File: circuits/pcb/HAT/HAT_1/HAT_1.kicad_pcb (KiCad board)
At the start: 2 copper layers, 75.4 x 55.9 mm, 11 parts, among them J1 Raspberry pi 5 GPIOs, J12 power input, J2 motor1, J3 motor1, J4 Conn_01x16_Pin, J5 motor2, J7 motor2, U1 ESP32-DEVKITC-32D, U2 L293D, U3 L293D

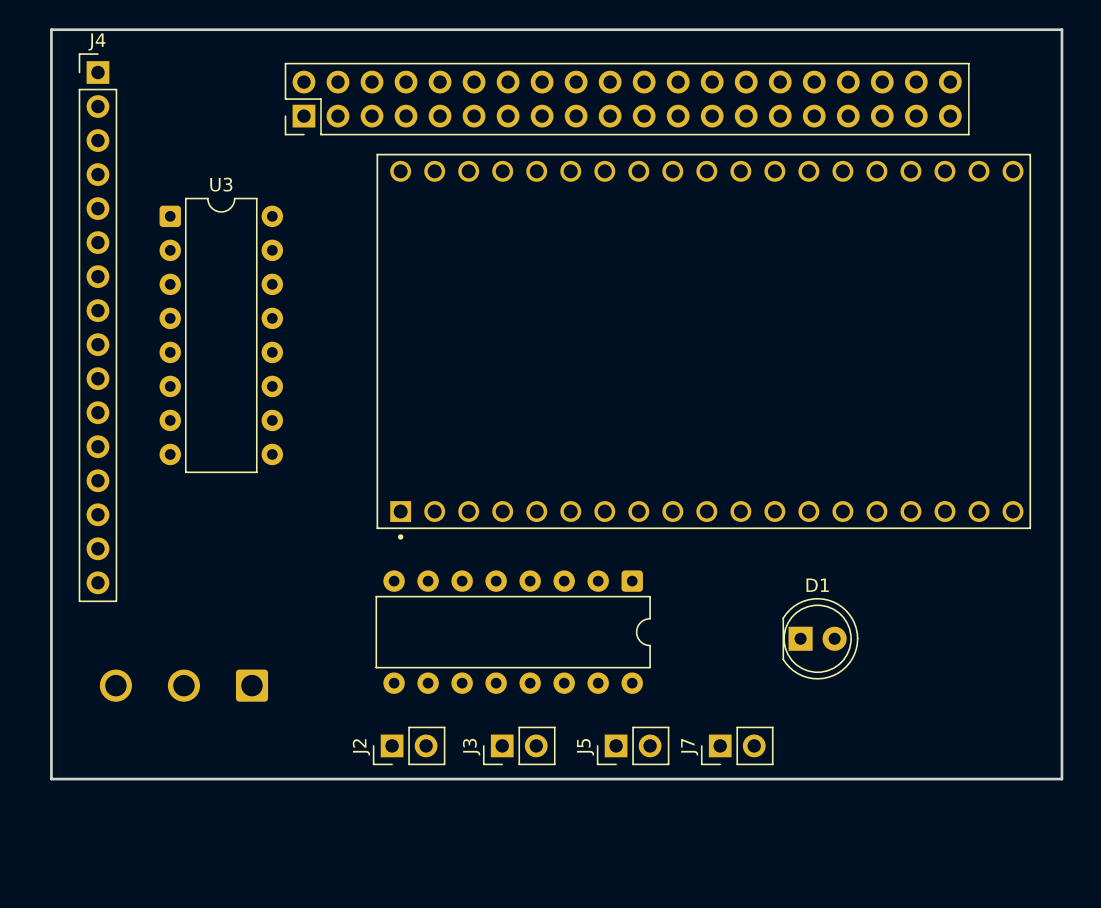
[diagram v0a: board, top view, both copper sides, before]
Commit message: ..
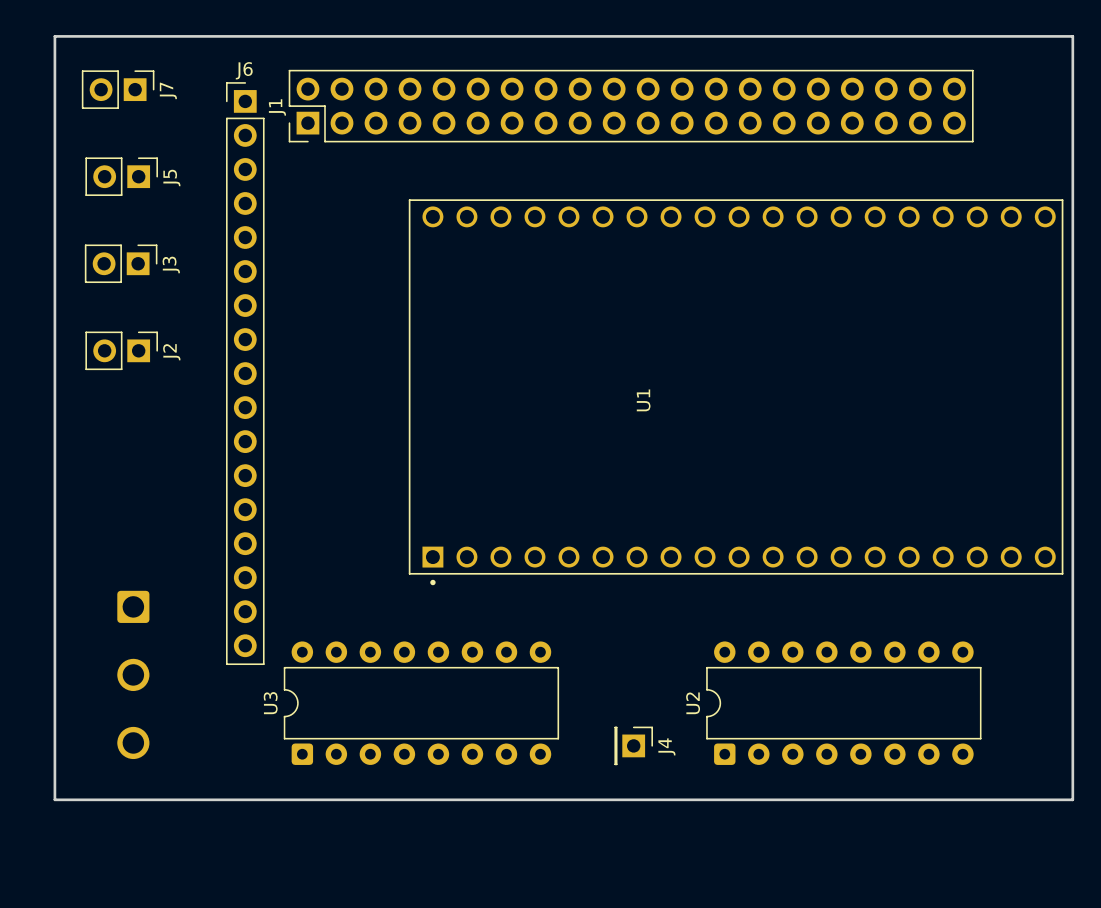
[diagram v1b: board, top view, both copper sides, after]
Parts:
- removed D1: LED, LED_THT:LED_D5.0mm
- added J6: Conn_01x17_Pin, Connector_PinHeader_2.54mm:PinHeader_1x17_P2.54mm_Vertical, F.Cu at (121.0, 79.9)
- J4: value Conn_01x16_Pin -> Conn_01x01_Pin; footprint Connector_PinHeader_2.54mm:PinHeader_1x16_P2.54mm_Vertical -> Connector_PinHeader_2.54mm:PinHeader_1x01_P2.54mm_Vertical
- moved J7 65.6 mm to (112.8, 79.0), turned to -90 degrees
- moved J4 64.2 mm to (150.0, 128.0), turned to -90 degrees
- moved J5 55.5 mm to (113.0, 85.5), turned to -90 degrees
- moved J3 45.1 mm to (113.0, 92.0), turned to -90 degrees
- moved U3 41.4 mm to (125.3, 128.6), turned to 90 degrees
- moved J2 35.0 mm to (113.0, 98.5), turned to -90 degrees
- moved U2 14.7 mm to (156.8, 128.6), turned to 90 degrees
- moved J12 10.6 mm to (112.6, 117.6), turned to -90 degrees
- moved U1 4.17 mm to (154.8, 101.2)
- moved J1 0.60 mm to (125.7, 81.5)
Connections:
- J4 pad 1: +5V -> Net-(J4-Pin_1)
- U1 pad J2-1: unconnected-(U1-3V3-PadJ2-1) -> Net-(J4-Pin_1)
- U1 pad J3-11: GPS RX -> TH_CAM SDA
- U1 pad J3-16: Net-(D1-A) -> TH_CAM SCL
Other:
- board size 75.4 x 55.9 mm -> 76 x 57 mm

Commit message: ...
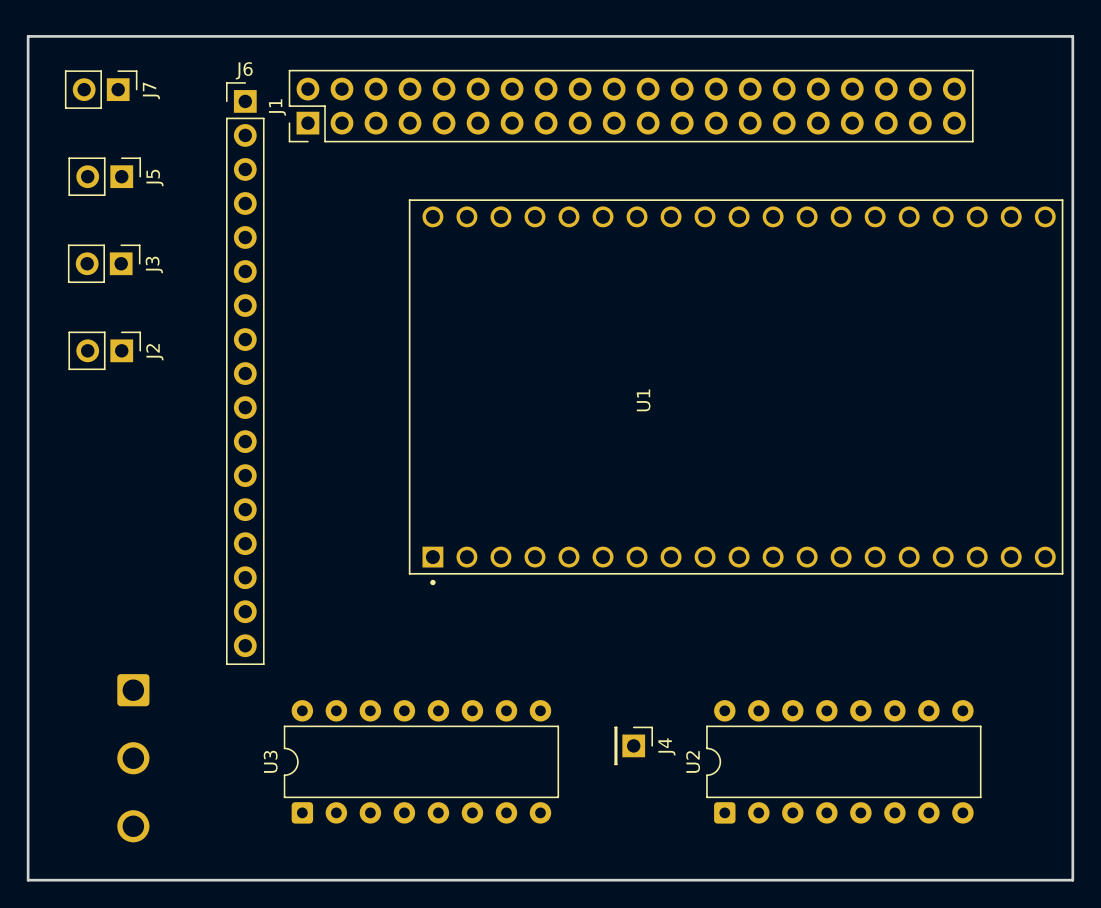
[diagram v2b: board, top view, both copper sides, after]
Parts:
- moved J12 6.22 mm to (112.6, 123.8)
- moved U2 4.38 mm to (156.8, 133.0)
- moved U3 4.38 mm to (125.3, 133.0)
- moved J2 1.27 mm to (111.8, 98.5)
- moved J3 1.27 mm to (111.7, 92.0)
- moved J5 1.27 mm to (111.8, 85.5)
- moved J7 1.27 mm to (111.5, 79.0)
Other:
- board size 76 x 57 mm -> 78 x 63 mm
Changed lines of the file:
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@@
 	(footprint "Package_DIP:DIP-16_W7.62mm"
 		(layer "F.Cu")
-		(at 156.8 128.62 90)
+		(at 156.8 133 90)
 		(descr "16-lead though-hole mounted DIP package, row spacing 7.62mm (300 mils)")
 		(tags "THT DIP DIL PDIP 2.54mm 7.62mm 300mil")
@@
 	(footprint "Connector_PinHeader_2.54mm:PinHeader_1x02_P2.54mm_Vertical"
 		(layer "F.Cu")
-		(at 113.04 85.5 -90)
+		(at 111.775 85.5 -90)
 		(descr "Through hole straight pin header, 1x02, 2.54mm pitch, single row")
 		(tags "Through hole pin header THT 1x02 2.54mm single row")
@@
 	(footprint "Connector_PinHeader_2.54mm:PinHeader_1x02_P2.54mm_Vertical"
 		(layer "F.Cu")
-		(at 113.04 98.5 -90)
+		(at 111.775 98.5 -90)
 		(descr "Through hole straight pin header, 1x02, 2.54mm pitch, single row")
 		(tags "Through hole pin header THT 1x02 2.54mm single row")
@@
 	(footprint "Package_DIP:DIP-16_W7.62mm"
 		(layer "F.Cu")
-		(at 125.26 128.62 90)
+		(at 125.26 133 90)
 		(descr "16-lead though-hole mounted DIP package, row spacing 7.62mm (300 mils)")
 		(tags "THT DIP DIL PDIP 2.54mm 7.62mm 300mil")
@@
 	(footprint "Connector_PinHeader_2.54mm:PinHeader_1x02_P2.54mm_Vertical"
 		(layer "F.Cu")
-		(at 112.775 79 -90)
+		(at 111.51 79 -90)
 		(descr "Through hole straight pin header, 1x02, 2.54mm pitch, single row")
 		(tags "Through hole pin header THT 1x02 2.54mm single row")
@@
 	(footprint "Connector_PinHeader_2.54mm:PinHeader_1x02_P2.54mm_Vertical"
 		(layer "F.Cu")
-		(at 113 92 -90)
+		(at 111.735 92 -90)
 		(descr "Through hole straight pin header, 1x02, 2.54mm pitch, single row")
 		(tags "Through hole pin header THT 1x02 2.54mm single row")
@@
 	(footprint "TerminalBlock_CUI:TerminalBlock_CUI_TB007-508-03_1x03_P5.08mm_Horizontal"
 		(layer "B.Cu")
-		(at 112.6425 117.62 -90)
+		(at 112.6425 123.84 -90)
 		(descr "Terminal Block CUI TB007-508-03, 3 pins, pitch 5.08mm, size 15.8x10.2mm, drill diameter 1.6mm, pad diameter 2.4mm, https://www.cuidevices.com/product/resource/tb007-508.pdf, script-generated using https://gitlab.com/kicad/libraries/kicad-footprint-generator/scripts/TerminalBlock_CUI")
 		(tags "THT Terminal Block CUI TB007-508-03 pitch 5.08mm size 15.8x10.2mm drill 1.6mm pad 2.4mm")
@@
 	)
 	(gr_rect
-		(start 106.785126 75.025126)
-		(end 182.785126 132.025126)
+		(start 104.785126 75.025126)
+		(end 182.785126 138.025126)
 		(stroke
 			(width 0.2)
@@
 		)
 		(fill no)
+		(locked yes)
 		(layer "Edge.Cuts")
 	)
